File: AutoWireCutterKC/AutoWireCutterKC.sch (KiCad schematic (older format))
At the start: 17 parts, among them J1 LCD I/O, J2 ISP, J3 LCD Serial, J5 LCD Power, J6 Servo, J8 Barrel_Jack, J9 Stepper, U1 ATMEGA328P-AU, U2 MCP1700_SOT23, U3 LT1129-5.0_SOT223

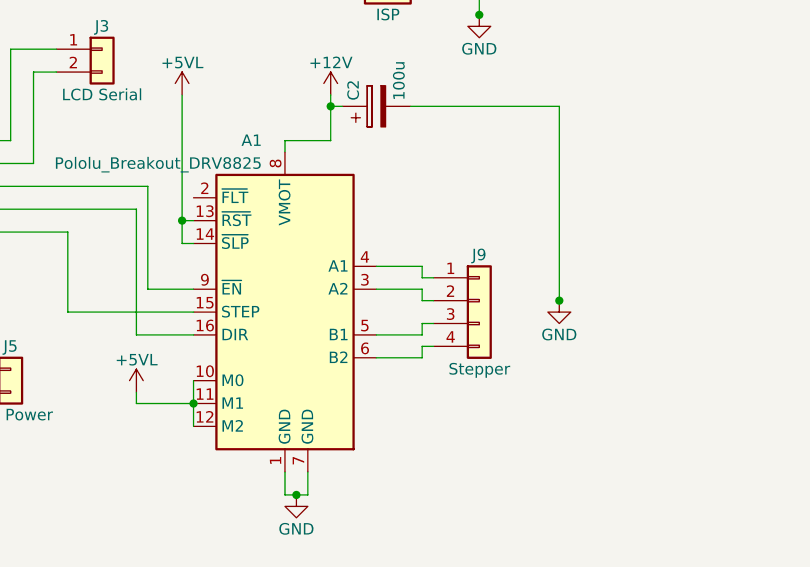
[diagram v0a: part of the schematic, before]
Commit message: Rewiring - Layout changed again...
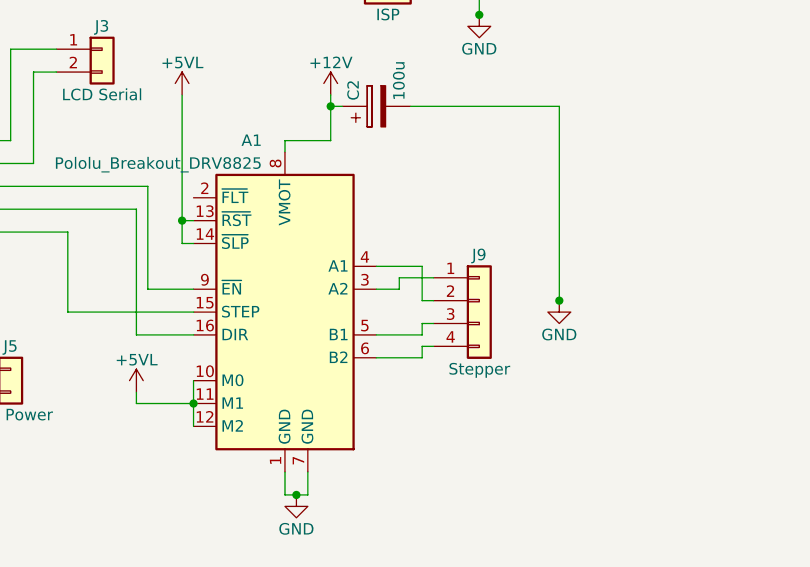
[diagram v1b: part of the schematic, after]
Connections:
- net at J9.1 (Pin_1): now also A1.3 (A2); no longer A1.4 (A1)
- net at J9.2 (Pin_2): now also A1.4 (A1); no longer A1.3 (A2)
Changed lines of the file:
@@
 $EndComp
 $Comp
-L GND #PWR02
+L GND #PWR01
 U 1 1 5B16A938
 P 1250 5050
-F 0 "#PWR02" H 1250 4800 50  0001 C CNN
+F 0 "#PWR01" H 1250 4800 50  0001 C CNN
 F 1 "GND" H 1250 4900 50  0000 C CNN
 F 2 "" H 1250 5050 50  0001 C CNN
@@
 $EndComp
 $Comp
-L GND #PWR03
+L GND #PWR02
 U 1 1 5B16B18B
 P 6600 3800
-F 0 "#PWR03" H 6600 3550 50  0001 C CNN
+F 0 "#PWR02" H 6600 3550 50  0001 C CNN
 F 1 "GND" H 6600 3650 50  0000 C CNN
 F 2 "" H 6600 3800 50  0001 C CNN
@@
 $EndComp
 $Comp
-L GND #PWR04
+L GND #PWR03
 U 1 1 5B18046F
 P 6950 5050
-F 0 "#PWR04" H 6950 4800 50  0001 C CNN
+F 0 "#PWR03" H 6950 4800 50  0001 C CNN
 F 1 "GND" H 6950 4900 50  0000 C CNN
 F 2 "" H 6950 5050 50  0001 C CNN
@@
 $EndComp
 $Comp
-L GND #PWR05
+L GND #PWR04
 U 1 1 5B1AA1E5
 P 4150 5500
-F 0 "#PWR05" H 4150 5250 50  0001 C CNN
+F 0 "#PWR04" H 4150 5250 50  0001 C CNN
 F 1 "GND" H 4150 5350 50  0000 C CNN
 F 2 "" H 4150 5500 50  0001 C CNN
@@
 $EndComp
 $Comp
-L +5V #PWR06
+L +5V #PWR05
 U 1 1 5B1AA79B
 P 3300 5500
-F 0 "#PWR06" H 3300 5350 50  0001 C CNN
+F 0 "#PWR05" H 3300 5350 50  0001 C CNN
 F 1 "+5V" H 3300 5640 50  0000 C CNN
 F 2 "" H 3300 5500 50  0001 C CNN
@@
 $EndComp
 $Comp
-L +12V #PWR07
+L +12V #PWR06
 U 1 1 5B1EB3CF
 P 9350 2800
-F 0 "#PWR07" H 9350 2650 50  0001 C CNN
+F 0 "#PWR06" H 9350 2650 50  0001 C CNN
 F 1 "+12V" H 9350 2940 50  0000 C CNN
 F 2 "" H 9350 2800 50  0001 C CNN
@@
 $EndComp
 $Comp
-L GND #PWR08
+L GND #PWR07
 U 1 1 5B1EB405
 P 9000 2800
-F 0 "#PWR08" H 9000 2550 50  0001 C CNN
+F 0 "#PWR07" H 9000 2550 50  0001 C CNN
 F 1 "GND" H 9000 2650 50  0000 C CNN
 F 2 "" H 9000 2800 50  0001 C CNN
@@
 $EndComp
 $Comp
-L GND #PWR09
+L GND #PWR08
 U 1 1 5B1EC3EE
 P 8950 4050
-F 0 "#PWR09" H 8950 3800 50  0001 C CNN
+F 0 "#PWR08" H 8950 3800 50  0001 C CNN
 F 1 "GND" H 8950 3900 50  0000 C CNN
 F 2 "" H 8950 4050 50  0001 C CNN
@@
 $EndComp
 $Comp
-L GND #PWR010
+L GND #PWR09
 U 1 1 5B1EC424
 P 8950 4850
-F 0 "#PWR010" H 8950 4600 50  0001 C CNN
+F 0 "#PWR09" H 8950 4600 50  0001 C CNN
 F 1 "GND" H 8950 4700 50  0000 C CNN
 F 2 "" H 8950 4850 50  0001 C CNN
@@
 $EndComp
 $Comp
-L +5V #PWR011
+L +5V #PWR010
 U 1 1 5B1EC45A
 P 9700 3650
-F 0 "#PWR011" H 9700 3500 50  0001 C CNN
+F 0 "#PWR010" H 9700 3500 50  0001 C CNN
 F 1 "+5V" H 9700 3790 50  0000 C CNN
 F 2 "" H 9700 3650 50  0001 C CNN
@@
 $EndComp
 $Comp
-L +12V #PWR012
+L +12V #PWR011
 U 1 1 5B1EC490
 P 8150 4450
-F 0 "#PWR012" H 8150 4300 50  0001 C CNN
+F 0 "#PWR011" H 8150 4300 50  0001 C CNN
 F 1 "+12V" H 8150 4590 50  0000 C CNN
 F 2 "" H 8150 4450 50  0001 C CNN
@@
 $EndComp
 $Comp
-L +12V #PWR013
+L +12V #PWR012
 U 1 1 5B1EC4C6
 P 8300 3650
-F 0 "#PWR013" H 8300 3500 50  0001 C CNN
+F 0 "#PWR012" H 8300 3500 50  0001 C CNN
 F 1 "+12V" H 8300 3790 50  0000 C CNN
 F 2 "" H 8300 3650 50  0001 C CNN
@@
 $EndComp
 $Comp
-L +5VL #PWR014
+L +5VL #PWR013
 U 1 1 5B1EDDCC
 P 4250 5150
-F 0 "#PWR014" H 4250 5000 50  0001 C CNN
+F 0 "#PWR013" H 4250 5000 50  0001 C CNN
 F 1 "+5VL" H 4250 5290 50  0000 C CNN
 F 2 "" H 4250 5150 50  0001 C CNN
@@
 $EndComp
 $Comp
-L +5VL #PWR015
+L +5VL #PWR014
 U 1 1 5B1EDE02
 P 1350 2750
-F 0 "#PWR015" H 1350 2600 50  0001 C CNN
+F 0 "#PWR014" H 1350 2600 50  0001 C CNN
 F 1 "+5VL" H 1350 2890 50  0000 C CNN
 F 2 "" H 1350 2750 50  0001 C CNN
@@
 $EndComp
 $Comp
-L +5VL #PWR016
+L +5VL #PWR015
 U 1 1 5B1EDFD3
 P 9600 4450
-F 0 "#PWR016" H 9600 4300 50  0001 C CNN
+F 0 "#PWR015" H 9600 4300 50  0001 C CNN
 F 1 "+5VL" H 9600 4590 50  0000 C CNN
 F 2 "" H 9600 4450 50  0001 C CNN
@@
 $EndComp
 $Comp
-L +12V #PWR017
+L +12V #PWR016
 U 1 1 5B1EE30F
 P 5950 4150
-F 0 "#PWR017" H 5950 4000 50  0001 C CNN
+F 0 "#PWR016" H 5950 4000 50  0001 C CNN
 F 1 "+12V" H 5950 4290 50  0000 C CNN
 F 2 "" H 5950 4150 50  0001 C CNN
@@
 $EndComp
 $Comp
-L GND #PWR018
+L GND #PWR017
 U 1 1 5B1F9E36
 P 5800 5900
-F 0 "#PWR018" H 5800 5650 50  0001 C CNN
+F 0 "#PWR017" H 5800 5650 50  0001 C CNN
 F 1 "GND" H 5800 5750 50  0000 C CNN
 F 2 "" H 5800 5900 50  0001 C CNN
@@
 Connection ~ 6450 3500
 Wire Wire Line
-	6150 4900 6350 4900
-Wire Wire Line
-	6350 4900 6350 4950
-Wire Wire Line
-	6350 4950 6400 4950
-Wire Wire Line
-	6150 5000 6350 5000
-Wire Wire Line
-	6350 5000 6350 5050
-Wire Wire Line
-	6350 5050 6400 5050
-Wire Wire Line
 	6150 5200 6350 5200
 Wire Wire Line
@@
 	5750 4350 5750 4400
 $Comp
-L +5VL #PWR019
+L +5VL #PWR018
 U 1 1 5B1FAD0F
 P 5100 5450
-F 0 "#PWR019" H 5100 5300 50  0001 C CNN
+F 0 "#PWR018" H 5100 5300 50  0001 C CNN
 F 1 "+5VL" H 5100 5590 50  0000 C CNN
 F 2 "" H 5100 5450 50  0001 C CNN
@@
 	9250 3650 9700 3650
 $Comp
-L +5VL #PWR020
+L +5VL #PWR019
 U 1 1 5B1FD55B
 P 5300 4150
-F 0 "#PWR020" H 5300 4000 50  0001 C CNN
+F 0 "#PWR019" H 5300 4000 50  0001 C CNN
 F 1 "+5VL" H 5300 4290 50  0000 C CNN
 F 2 "" H 5300 4150 50  0001 C CNN
@@
 	3850 6100 3900 6100
 $Comp
-L +5VL #PWR?
+L +5VL #PWR020
 U 1 1 5B212B86
 P 6150 3200
-F 0 "#PWR?" H 6150 3050 50  0001 C CNN
+F 0 "#PWR020" H 6150 3050 50  0001 C CNN
 F 1 "+5VL" H 6150 3340 50  0000 C CNN
 F 2 "" H 6150 3200 50  0001 C CNN
@@
 	0    -1   -1   0
 $EndComp
+Wire Wire Line
+	6150 5000 6250 5000
+Wire Wire Line
+	6250 5000 6250 4950
+Wire Wire Line
+	6250 4950 6400 4950
+Wire Wire Line
+	6150 4900 6350 4900
+Wire Wire Line
+	6350 4900 6350 5050
+Wire Wire Line
+	6350 5050 6400 5050
 $EndSCHEMATC
